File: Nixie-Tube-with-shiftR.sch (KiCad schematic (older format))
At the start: 51 parts, among them J1 Conn_01x05_Male, J2 Conn_01x01_Female, J3 Conn_01x05_Female, J4 Conn_01x01_Male, Q1 MMBTA42LT1, Q10 MMBTA42LT1, Q11 AO3400, Q12 AO3400, Q13 AO3400, Q14 MMBTA42LT1, Q2 MMBTA42LT1, Q3 MMBTA42LT1, Q4 MMBTA42LT1, Q5 MMBTA42LT1, Q6 MMBTA42LT1, Q7 MMBTA42LT1, Q8 MMBTA42LT1, Q9 MMBTA42LT1, U1 74HC595D, U2 nixie-tube, U3 74HC595D, U4 ams1117-5.0

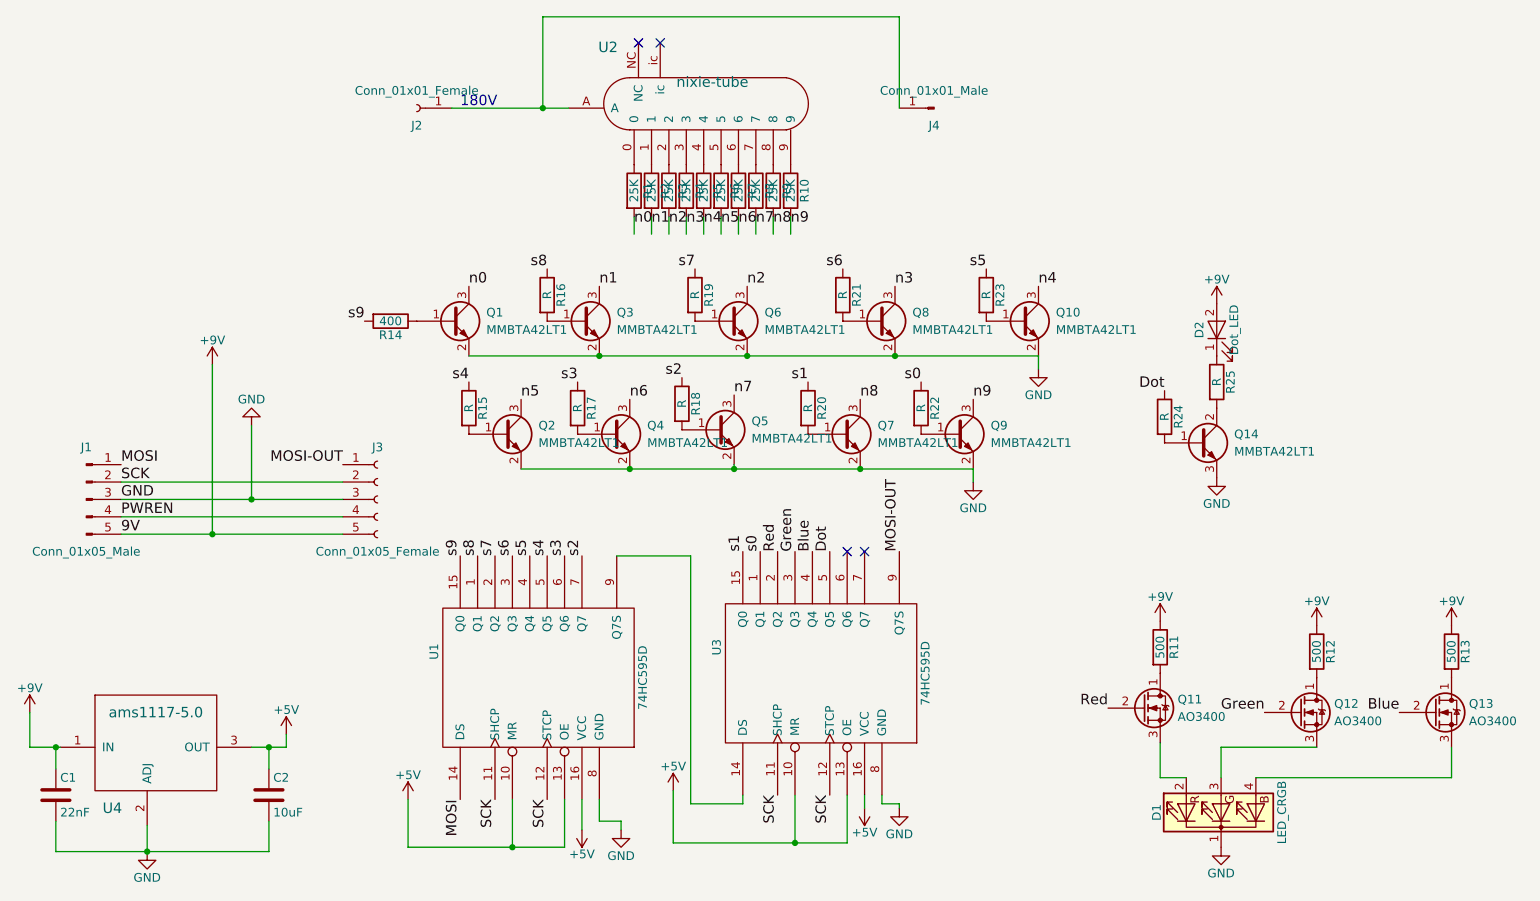
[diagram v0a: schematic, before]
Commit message: placed all the component
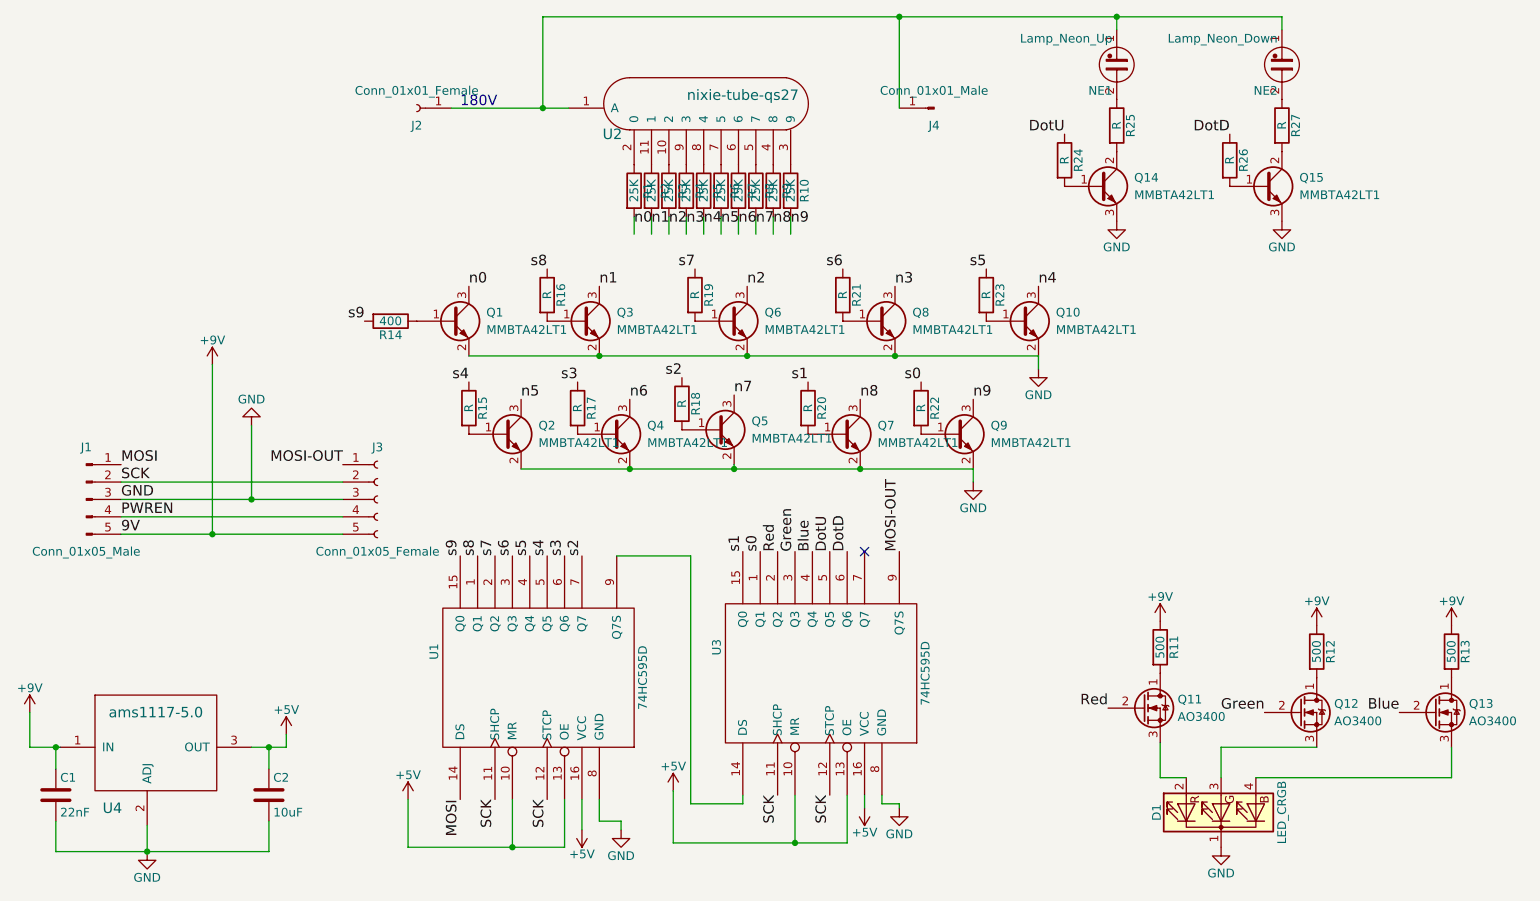
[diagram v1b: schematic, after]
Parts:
- removed D2: Dot_LED, symbol LED-RESCUE-Nixie-Tube-with-shiftR
- removed U2: nixie-tube, nixie-tube-fp:qs30-1, symbol nixie-tube
- added NE1: Lamp_Neon_Up, nixie-tube-fp:neon-tube, symbol Lamp_Neon
- added NE2: Lamp_Neon_Down, nixie-tube-fp:neon-tube, symbol Lamp_Neon
- added Q15: MMBTA42LT1, TO_SOT_Packages_SMD:SOT-23, symbol Q_NPN_BCE
- added R26, R27: R, Resistors_SMD:R_0603, symbol R
- added U2: nixie-tube-qs27, nixie-tube-fp:qs27-1, symbol nixie-tube-qs27
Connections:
- net labels added: DotD, DotU
- net labels removed: Dot
- wire segments 61 -> 63
- no-connect marks 4 -> 1
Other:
- moved on the sheet: Q14, R24, R25
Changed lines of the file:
@@
 Comment4 ""
 $EndDescr
-$Comp
-L nixie-tube U2
-U 1 1 59DE1F0A
-P 5450 1950
-F 0 "U2" H 4850 2550 60  0000 C CNN
-F 1 "nixie-tube" H 5450 2350 60  0000 C CNN
-F 2 "nixie-tube-fp:qs30-1" H 5150 1950 60  0001 C CNN
-F 3 "" H 5150 1950 60  0001 C CNN
-	1    5450 1950
-	1    0    0    -1
-$EndComp
 Text Notes 4000 1700 0    60   ~ 0
 180V
@@
 Wire Wire Line
 	6525 5700 6525 5725
-NoConn ~ 6225 4250
 NoConn ~ 6325 4250
 $Comp
@@
 	1    0    0    -1
 $EndComp
-NoConn ~ 5025 1325
-NoConn ~ 5150 1325
 $Comp
 L Conn_01x01_Female J2
@@
 MOSI-OUT
 $Comp
-L LED-RESCUE-Nixie-Tube-with-shiftR D2
-U 1 1 59E02618
-P 8350 2975
-F 0 "D2" H 8350 3075 50  0000 C CNN
-F 1 "Dot_LED" H 8350 2875 50  0000 C CNN
-F 2 "" H 8350 2975 50  0001 C CNN
-F 3 "" H 8350 2975 50  0001 C CNN
-	1    8350 2975
-	0    -1   -1   0
-$EndComp
-$Comp
 L Q_NPN_BCE Q14
 U 1 1 59E02747
-P 8250 3625
-F 0 "Q14" H 8450 3675 50  0000 L CNN
-F 1 "MMBTA42LT1" H 8450 3575 50  0000 L CNN
-F 2 "TO_SOT_Packages_SMD:SOT-23" H 8450 3725 50  0001 C CNN
-F 3 "" H 8250 3625 50  0001 C CNN
-	1    8250 3625
+P 7675 2150
+F 0 "Q14" H 7875 2200 50  0000 L CNN
+F 1 "MMBTA42LT1" H 7875 2100 50  0000 L CNN
+F 2 "TO_SOT_Packages_SMD:SOT-23" H 7875 2250 50  0001 C CNN
+F 3 "" H 7675 2150 50  0001 C CNN
+	1    7675 2150
 	1    0    0    -1
 $EndComp
@@
 L R R24
 U 1 1 59E037C1
-P 8050 3475
-F 0 "R24" V 8130 3475 50  0000 C CNN
-F 1 "R" V 8050 3475 50  0000 C CNN
-F 2 "Resistors_SMD:R_0603" V 7980 3475 50  0001 C CNN
-F 3 "" H 8050 3475 50  0001 C CNN
-	1    8050 3475
+P 7475 2000
+F 0 "R24" V 7555 2000 50  0000 C CNN
+F 1 "R" V 7475 2000 50  0000 C CNN
+F 2 "Resistors_SMD:R_0603" V 7405 2000 50  0001 C CNN
+F 3 "" H 7475 2000 50  0001 C CNN
+	1    7475 2000
 	1    0    0    -1
 $EndComp
 Text Label 6125 4250 1    60   ~ 0
-Dot
-Text Label 8050 3325 2    60   ~ 0
-Dot
+DotU
+Text Label 7475 1850 2    60   ~ 0
+DotU
 $Comp
 L GND #PWR06
 U 1 1 59E03A8E
-P 8350 3825
-F 0 "#PWR06" H 8350 3575 50  0001 C CNN
-F 1 "GND" H 8350 3675 50  0000 C CNN
-F 2 "" H 8350 3825 50  0001 C CNN
-F 3 "" H 8350 3825 50  0001 C CNN
-	1    8350 3825
+P 7775 2350
+F 0 "#PWR06" H 7775 2100 50  0001 C CNN
+F 1 "GND" H 7775 2200 50  0000 C CNN
+F 2 "" H 7775 2350 50  0001 C CNN
+F 3 "" H 7775 2350 50  0001 C CNN
+	1    7775 2350
 	1    0    0    -1
 $EndComp
@@
 L R R25
 U 1 1 59E03B9C
-P 8350 3275
-F 0 "R25" V 8430 3275 50  0000 C CNN
-F 1 "R" V 8350 3275 50  0000 C CNN
-F 2 "Resistors_SMD:R_0603" V 8280 3275 50  0001 C CNN
-F 3 "" H 8350 3275 50  0001 C CNN
-	1    8350 3275
+P 7775 1800
+F 0 "R25" V 7855 1800 50  0000 C CNN
+F 1 "R" V 7775 1800 50  0000 C CNN
+F 2 "Resistors_SMD:R_0603" V 7705 1800 50  0001 C CNN
+F 3 "" H 7775 1800 50  0001 C CNN
+	1    7775 1800
 	1    0    0    -1
 $EndComp
@@
 	1    0    0    -1
 $EndComp
-$Comp
-L +9V #PWR012
-U 1 1 59E167E2
-P 8350 2825
-F 0 "#PWR012" H 8350 2675 50  0001 C CNN
-F 1 "+9V" H 8350 2965 50  0000 C CNN
-F 2 "" H 8350 2825 50  0001 C CNN
-F 3 "" H 8350 2825 50  0001 C CNN
-	1    8350 2825
-	1    0    0    -1
-$EndComp
 Text Label 5000 2375 0    60   ~ 0
 n0
@@
 	4475 1700 4475 1175
 Wire Wire Line
-	4475 1175 6525 1175
+	4475 1175 8725 1175
 Wire Wire Line
 	6525 1175 6525 1700
@@
 $EndComp
 $Comp
-L +9V #PWR013
+L +9V #PWR012
 U 1 1 59E0CD5E
 P 1525 5175
-F 0 "#PWR013" H 1525 5025 50  0001 C CNN
+F 0 "#PWR012" H 1525 5025 50  0001 C CNN
 F 1 "+9V" H 1525 5315 50  0000 C CNN
 F 2 "" H 1525 5175 50  0001 C CNN
@@
 	1525 5375 1700 5375
 $Comp
-L +5V #PWR014
+L +5V #PWR013
 U 1 1 59E0CEE2
 P 3000 5300
-F 0 "#PWR014" H 3000 5150 50  0001 C CNN
+F 0 "#PWR013" H 3000 5150 50  0001 C CNN
 F 1 "+5V" H 3000 5440 50  0000 C CNN
 F 2 "" H 3000 5300 50  0001 C CNN
@@
 	3000 5375 3000 5300
 $Comp
-L GND #PWR015
+L GND #PWR014
 U 1 1 59E0CFCB
 P 2200 5975
-F 0 "#PWR015" H 2200 5725 50  0001 C CNN
+F 0 "#PWR014" H 2200 5725 50  0001 C CNN
 F 1 "GND" H 2200 5825 50  0000 C CNN
 F 2 "" H 2200 5975 50  0001 C CNN
@@
 	2200 5825 2200 5975
 $Comp
-L +5V #PWR016
+L +5V #PWR015
 U 1 1 59E0E450
 P 3700 5675
-F 0 "#PWR016" H 3700 5525 50  0001 C CNN
+F 0 "#PWR015" H 3700 5525 50  0001 C CNN
 F 1 "+5V" H 3700 5815 50  0000 C CNN
 F 2 "" H 3700 5675 50  0001 C CNN
@@
 $EndComp
 $Comp
-L +5V #PWR017
+L +5V #PWR016
 U 1 1 59E0E605
 P 4700 5850
-F 0 "#PWR017" H 4700 5700 50  0001 C CNN
+F 0 "#PWR016" H 4700 5700 50  0001 C CNN
 F 1 "+5V" H 4700 5990 50  0000 C CNN
 F 2 "" H 4700 5850 50  0001 C CNN
@@
 $EndComp
 $Comp
-L +5V #PWR018
+L +5V #PWR017
 U 1 1 59E0EA7E
 P 5225 5625
-F 0 "#PWR018" H 5225 5475 50  0001 C CNN
+F 0 "#PWR017" H 5225 5475 50  0001 C CNN
 F 1 "+5V" H 5225 5765 50  0000 C CNN
 F 2 "" H 5225 5625 50  0001 C CNN
@@
 $EndComp
 $Comp
-L +5V #PWR019
+L +5V #PWR018
 U 1 1 59E0EB56
 P 6325 5725
-F 0 "#PWR019" H 6325 5575 50  0001 C CNN
+F 0 "#PWR018" H 6325 5575 50  0001 C CNN
 F 1 "+5V" H 6325 5865 50  0000 C CNN
 F 2 "" H 6325 5725 50  0001 C CNN
@@
 	-1   0    0    1
 $EndComp
+$Comp
+L nixie-tube-qs27 U2
+U 1 1 59E1ACBC
+P 5450 1950
+F 0 "U2" H 4875 2050 60  0000 C CNN
+F 1 "nixie-tube-qs27" H 5625 2275 60  0000 C CNN
+F 2 "nixie-tube-fp:qs27-1" H 5150 1975 60  0001 C CNN
+F 3 "" H 5150 1975 60  0001 C CNN
+	1    5450 1950
+	1    0    0    -1
+$EndComp
+Wire Wire Line
+	7775 1175 7775 1250
+Connection ~ 6525 1175
+$Comp
+L Q_NPN_BCE Q15
+U 1 1 59E1EE85
+P 8625 2150
+F 0 "Q15" H 8825 2200 50  0000 L CNN
+F 1 "MMBTA42LT1" H 8825 2100 50  0000 L CNN
+F 2 "TO_SOT_Packages_SMD:SOT-23" H 8825 2250 50  0001 C CNN
+F 3 "" H 8625 2150 50  0001 C CNN
+	1    8625 2150
+	1    0    0    -1
+$EndComp
+$Comp
+L R R26
+U 1 1 59E1EE8B
+P 8425 2000
+F 0 "R26" V 8505 2000 50  0000 C CNN
+F 1 "R" V 8425 2000 50  0000 C CNN
+F 2 "Resistors_SMD:R_0603" V 8355 2000 50  0001 C CNN
+F 3 "" H 8425 2000 50  0001 C CNN
+	1    8425 2000
+	1    0    0    -1
+$EndComp
+Text Label 8425 1850 2    60   ~ 0
+DotD
+$Comp
+L GND #PWR019
+U 1 1 59E1EE92
+P 8725 2350
+F 0 "#PWR019" H 8725 2100 50  0001 C CNN
+F 1 "GND" H 8725 2200 50  0000 C CNN
+F 2 "" H 8725 2350 50  0001 C CNN
+F 3 "" H 8725 2350 50  0001 C CNN
+	1    8725 2350
+	1    0    0    -1
+$EndComp
+$Comp
+L R R27
+U 1 1 59E1EE98
+P 8725 1800
+F 0 "R27" V 8805 1800 50  0000 C CNN
+F 1 "R" V 8725 1800 50  0000 C CNN
+F 2 "Resistors_SMD:R_0603" V 8655 1800 50  0001 C CNN
+F 3 "" H 8725 1800 50  0001 C CNN
+	1    8725 1800
+	1    0    0    -1
+$EndComp
+Wire Wire Line
+	8725 1175 8725 1250
+Connection ~ 7775 1175
+$Comp
+L Lamp_Neon NE1
+U 1 1 59E2014E
+P 7775 1450
+F 0 "NE1" H 7800 1600 50  0000 L CNN
+F 1 "Lamp_Neon_Up" H 7800 1300 50  0000 L CNN
+F 2 "nixie-tube-fp:neon-tube" V 7775 1550 50  0001 C CNN
+F 3 "" V 7775 1550 50  0001 C CNN
+	1    7775 1450
+	-1   0    0    1
+$EndComp
+$Comp
+L Lamp_Neon NE2
+U 1 1 59E20B86
+P 8725 1450
+F 0 "NE2" H 8750 1600 50  0000 L CNN
+F 1 "Lamp_Neon_Down" H 8750 1300 50  0000 L CNN
+F 2 "nixie-tube-fp:neon-tube" V 8725 1550 50  0001 C CNN
+F 3 "" V 8725 1550 50  0001 C CNN
+	1    8725 1450
+	-1   0    0    1
+$EndComp
+Text Label 6225 4250 1    60   ~ 0
+DotD
 $EndSCHEMATC
